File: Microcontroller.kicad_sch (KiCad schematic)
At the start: 36 parts, among them SW1 Pairing, SW2 Add 10 BTH, U1 ESP32-S3-N16R8-Module, U13 PCA9557PW, U14 PCA9557PW, U2 PCA9557PW, U3 PCA9557PW

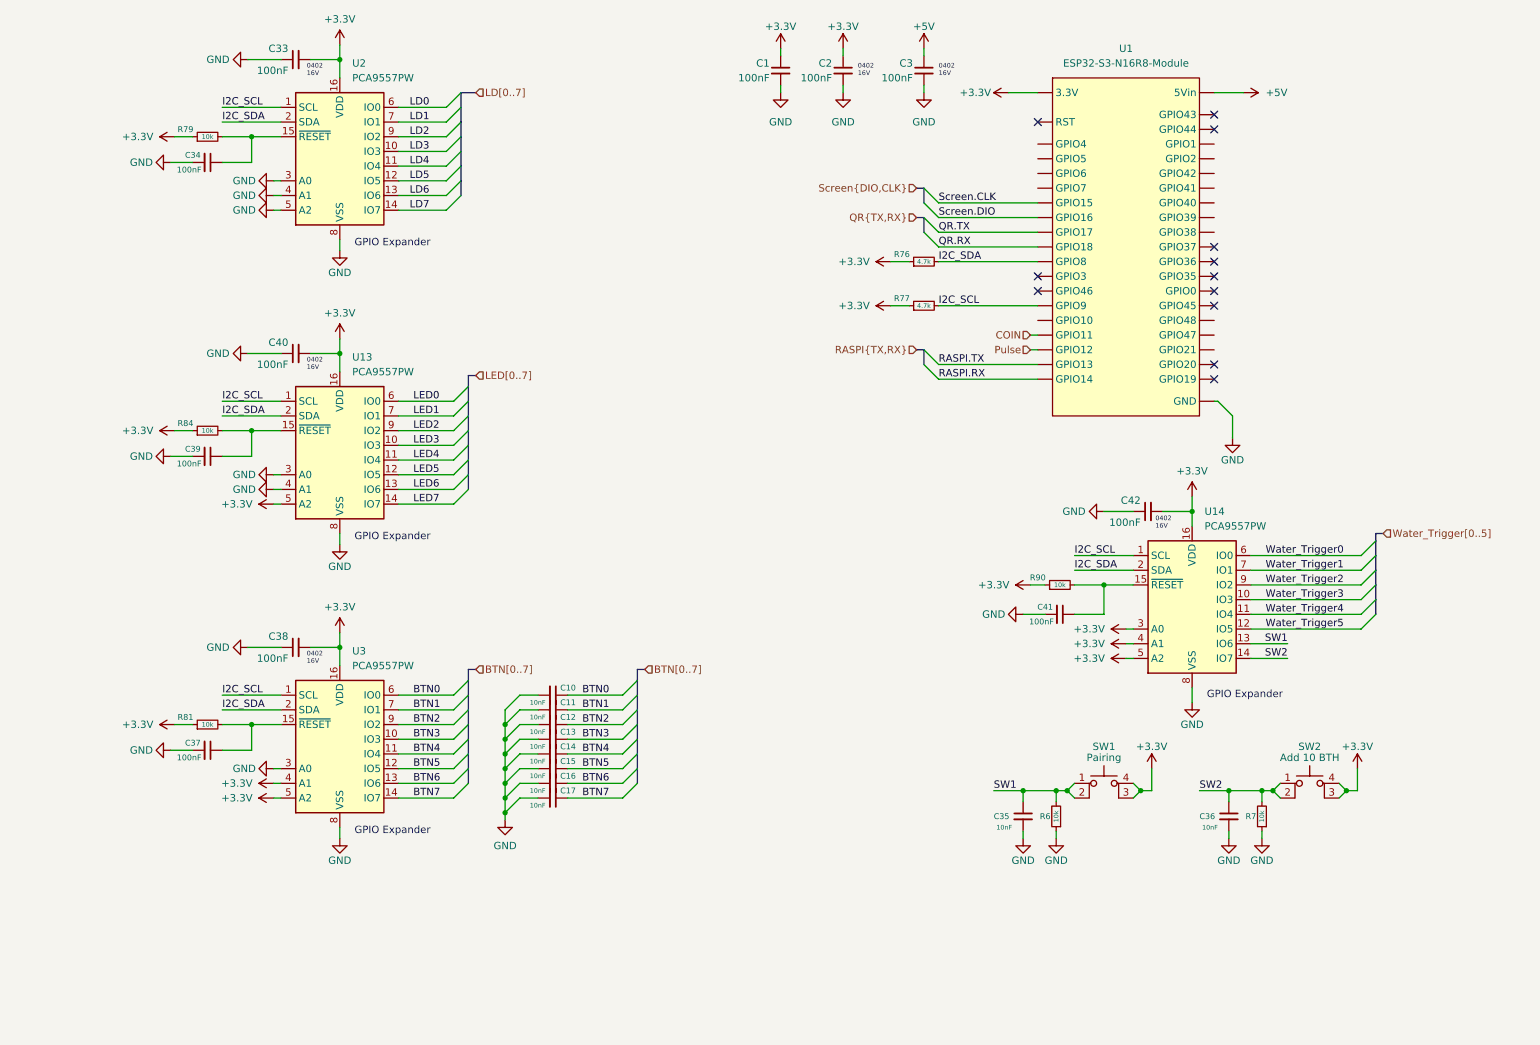
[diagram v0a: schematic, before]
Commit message: SCH finish
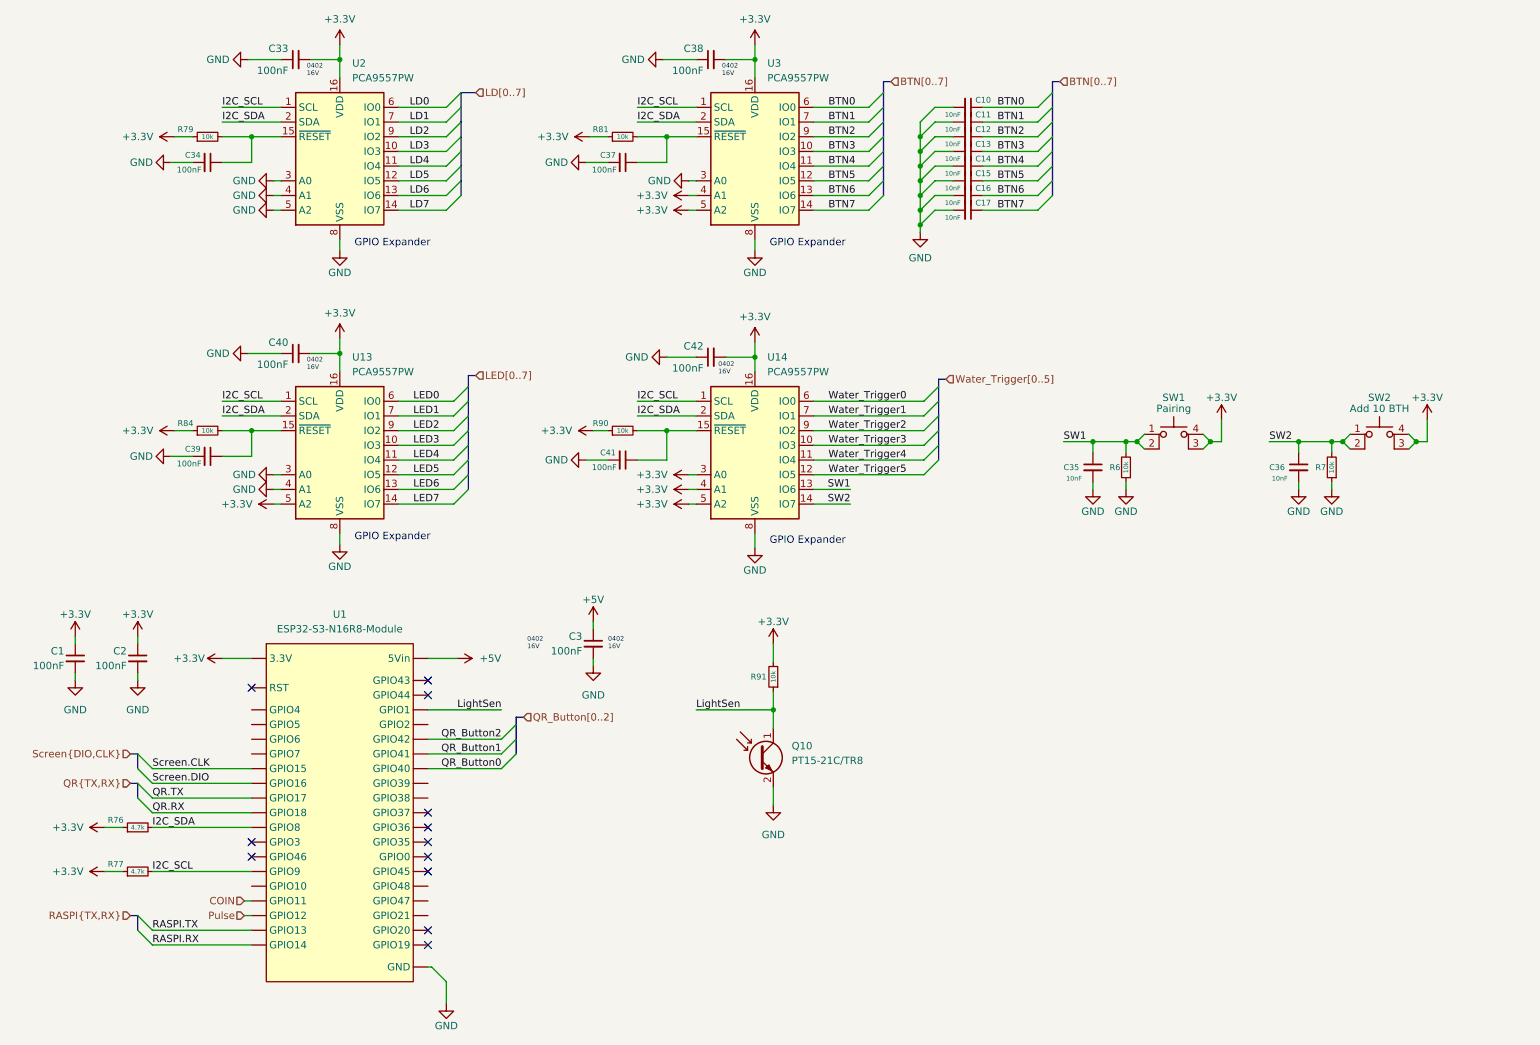
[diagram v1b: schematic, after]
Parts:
- added Q10: PT15-21C/TR8, LED_SMD:LED_1206_3216Metric, symbol Sensor_Optical:BPW42
- added R91: 10k, Resistor_SMD:R_0402_1005Metric, symbol Device:R_Small
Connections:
- net +3.3V: now also R91.2
- net GND: now also Q10.2 (E)
- net QR_Button0: now reaches U1.37 (GPIO40)
- net QR_Button1: now reaches U1.38 (GPIO41)
- net QR_Button2: now reaches U1.39 (GPIO42)
- net LightSen: now reaches U1.41 (GPIO1)
- net LightSen: now also Q10.1 (C), R91.1
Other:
- moved on the sheet: C1, C10, C11, C12, C13, C14, C15, C16, C17, C2, C3, C35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
